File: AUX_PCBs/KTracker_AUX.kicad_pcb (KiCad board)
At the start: 2 copper layers, 49.9 x 19.4 mm, 14 parts, among them J2 Conn_01x04_Female, U1 ME6211C, U9 MPU-9250

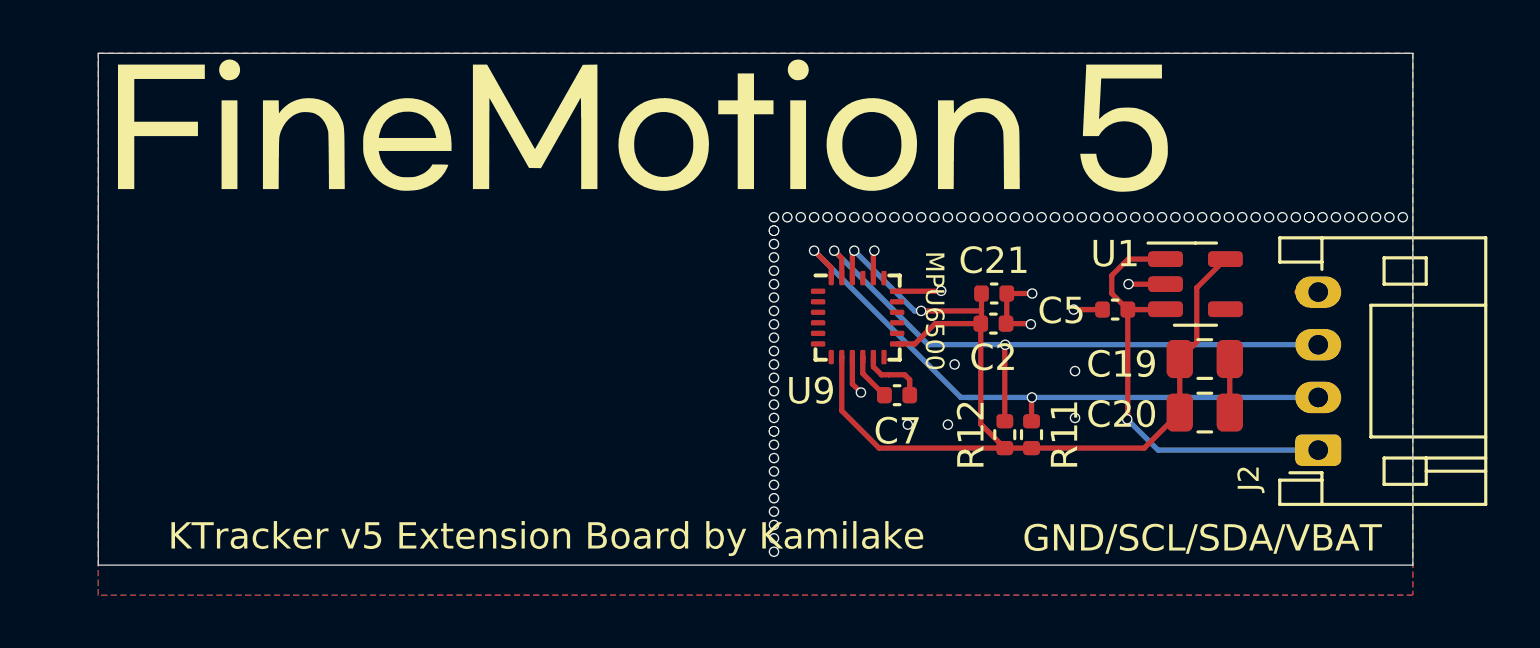
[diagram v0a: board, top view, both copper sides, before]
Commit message: .
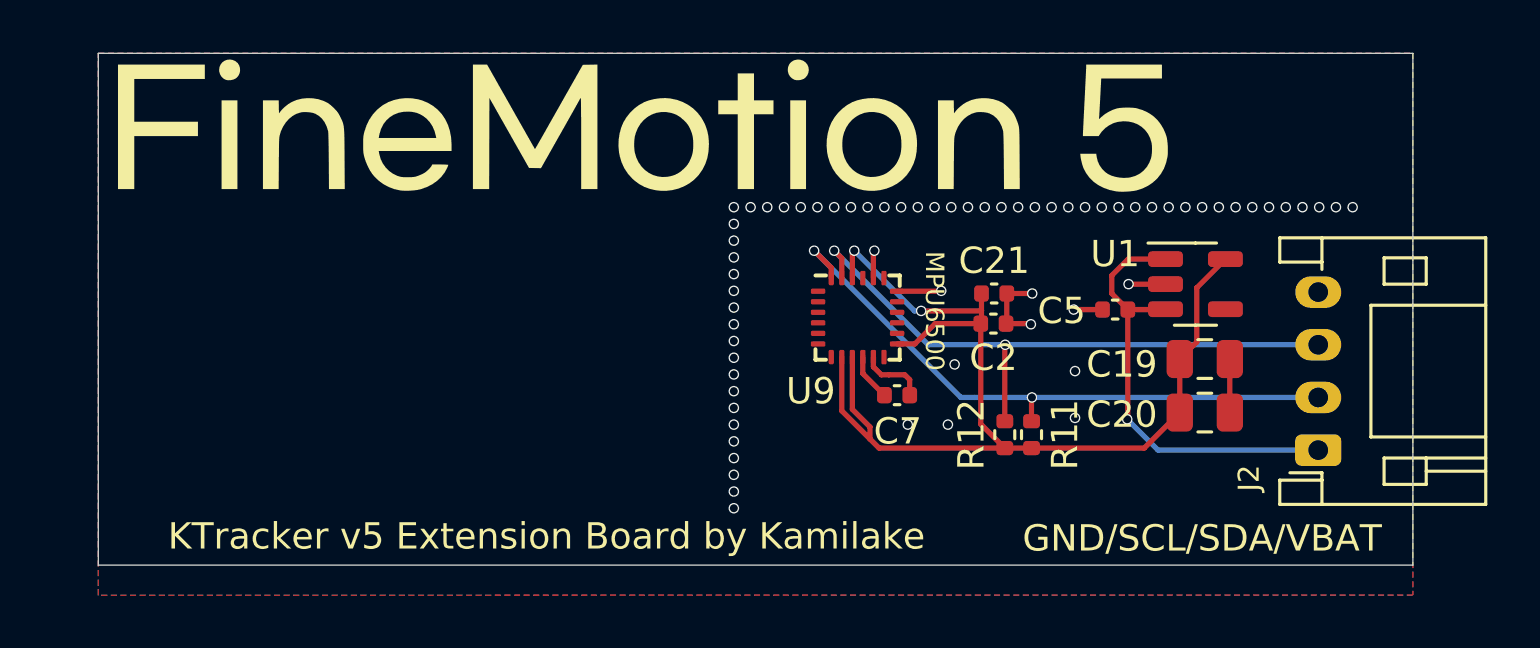
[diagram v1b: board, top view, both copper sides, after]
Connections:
- U9 pad 21: AUX_SDA -> unconnected-(U9-Pad21)
- U9 pad 7: AUX_SCL -> unconnected-(U9-Pad7)
- U9 pad 9: GND -> +3V3
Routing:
- net +3V3: track 39.2 -> 42.5 mm
- net GND: track 15.7 -> 13.5 mm, vias 88 -> 67
